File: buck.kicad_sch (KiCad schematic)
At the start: 8 parts, among them U7 DIO6012BCST6

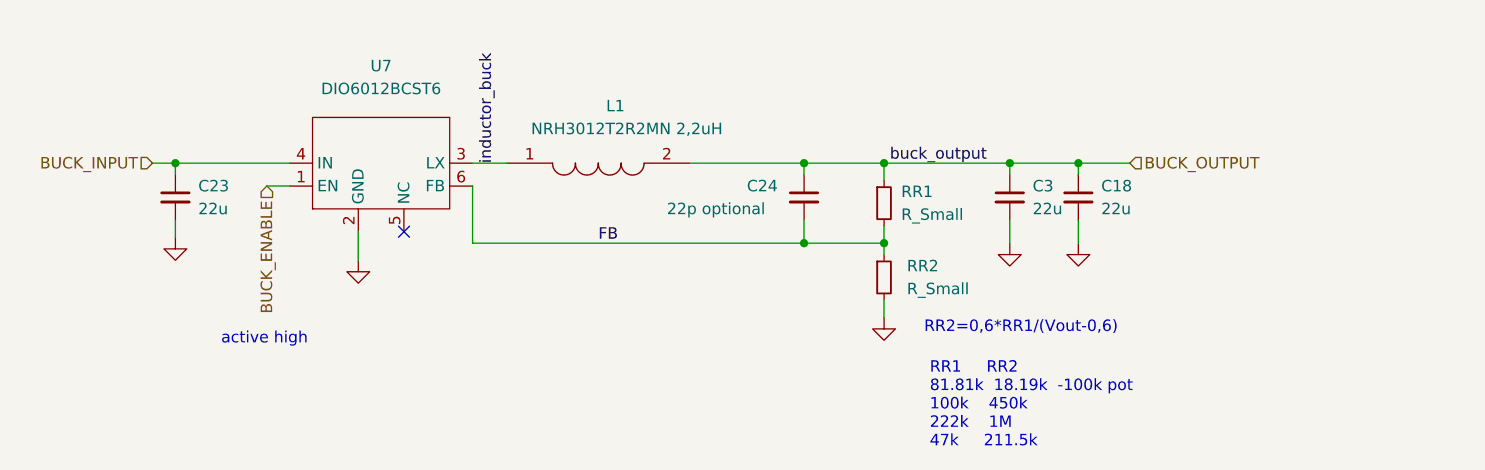
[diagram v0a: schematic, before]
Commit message: j
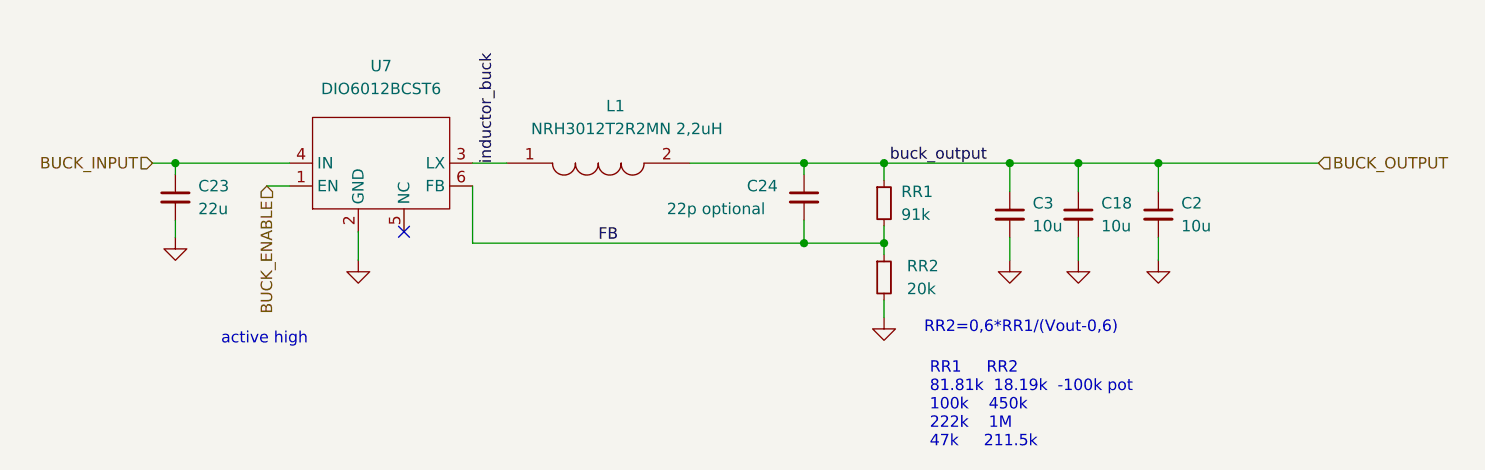
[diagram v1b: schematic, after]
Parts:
- added C2: 10u, Capacitor_SMD:C_0805_2012Metric, symbol Device:C_Small
- C18, C3: value 22u -> 10u; footprint Capacitor_THT:CP_Radial_D5.0mm_P2.00mm -> Capacitor_SMD:C_0805_2012Metric
- RR1: value R_Small -> 91k; footprint Resistor_THT:R_Axial_DIN0204_L3.6mm_D1.6mm_P5.08mm_Vertical -> Resistor_SMD:R_0805_2012Metric
- RR2: value R_Small -> 20k; footprint Resistor_THT:R_Axial_DIN0204_L3.6mm_D1.6mm_P5.08mm_Vertical -> Resistor_SMD:R_0805_2012Metric
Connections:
- net BUCK_OUTPUT: now also C2.1
- net GND: now also C2.2
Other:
- moved on the sheet: C18, C3
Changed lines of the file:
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@@
   (junction (at 83.82 59.69) (diameter 0) (color 0 0 0 0)
+  )
+  (junction (at 193.04 59.69) (diameter 0) (color 0 0 0 0)
   )
   (junction (at 162.56 59.69) (diameter 0) (color 0 0 0 0)
@@
     (stroke (width 0) (type default) (color 0 0 0 0))
   )
-  (wire (pts (xy 184.15 59.69) (xy 184.15 60.96))
+  (wire (pts (xy 184.15 59.69) (xy 184.15 62.865))
     (stroke (width 0) (type default) (color 0 0 0 0))
   )
@@
     (stroke (width 0) (type default) (color 0 0 0 0))
   )
+  (wire (pts (xy 193.04 59.69) (xy 210.82 59.69))
+    (stroke (width 0) (type default) (color 0 0 0 0))
+  )
   (wire (pts (xy 153.67 68.58) (xy 162.56 68.58))
     (stroke (width 0) (type default) (color 0 0 0 0))
   )
-  (wire (pts (xy 176.53 66.04) (xy 176.53 68.58))
+  (wire (pts (xy 176.53 67.945) (xy 176.53 70.485))
     (stroke (width 0) (type default) (color 0 0 0 0))
   )
@@
     (stroke (width 0) (type default) (color 0 0 0 0))
   )
-  (wire (pts (xy 184.15 59.69) (xy 189.865 59.69))
+  (wire (pts (xy 184.15 59.69) (xy 193.04 59.69))
     (stroke (width 0) (type default) (color 0 0 0 0))
   )
@@
     (stroke (width 0) (type default) (color 0 0 0 0))
   )
-  (wire (pts (xy 176.53 59.69) (xy 176.53 60.96))
+  (wire (pts (xy 176.53 59.69) (xy 176.53 62.865))
     (stroke (width 0) (type default) (color 0 0 0 0))
   )
@@
     (stroke (width 0) (type default) (color 0 0 0 0))
   )
+  (wire (pts (xy 193.04 67.945) (xy 193.04 70.485))
+    (stroke (width 0) (type default) (color 0 0 0 0))
+  )
+  (wire (pts (xy 193.04 59.69) (xy 193.04 62.865))
+    (stroke (width 0) (type default) (color 0 0 0 0))
+  )
   (wire (pts (xy 104.14 67.31) (xy 104.14 70.485))
     (stroke (width 0) (type default) (color 0 0 0 0))
@@
     (stroke (width 0) (type default) (color 0 0 0 0))
   )
-  (wire (pts (xy 184.15 66.04) (xy 184.15 68.58))
+  (wire (pts (xy 184.15 67.945) (xy 184.15 70.485))
     (stroke (width 0) (type default) (color 0 0 0 0))
   )
@@
     (effects (font (size 1.27 1.27)) (justify right))
   )
-  (hierarchical_label "BUCK_OUTPUT" (shape input) (at 189.865 59.69 0)
+  (hierarchical_label "BUCK_OUTPUT" (shape input) (at 210.82 59.69 0)
     (effects (font (size 1.27 1.27)) (justify left))
   )
@@
       (effects (font (size 1.27 1.27)) (justify left))
     )
-    (property "Value" "R_Small" (id 1) (at 165.1 73.6599 0)
-      (effects (font (size 1.27 1.27)) (justify left))
-    )
-    (property "Footprint" "Resistor_THT:R_Axial_DIN0204_L3.6mm_D1.6mm_P5.08mm_Vertical" (id 2) (at 162.56 72.39 0)
+    (property "Value" "20k" (id 1) (at 165.1 73.6599 0)
+      (effects (font (size 1.27 1.27)) (justify left))
+    )
+    (property "Footprint" "Resistor_SMD:R_0805_2012Metric" (id 2) (at 162.56 72.39 0)
       (effects (font (size 1.27 1.27)) hide)
     )
@@
     (pin "1")
   )
-  (symbol (lib_id "power:GND") (at 184.15 68.58 0) (unit 1)
-    (in_bom yes) (on_board yes) (fields_autoplaced)
-    (property "Reference" "#PWR0104" (id 0) (at 184.15 74.93 0)
-      (effects (font (size 1.27 1.27)) hide)
-    )
-    (property "Value" "GND" (id 1) (at 184.15 73.66 0)
-      (effects (font (size 1.27 1.27)) hide)
-    )
-    (property "Footprint" "" (id 2) (at 184.15 68.58 0)
-      (effects (font (size 1.27 1.27)) hide)
-    )
-    (property "Datasheet" "" (id 3) (at 184.15 68.58 0)
+  (symbol (lib_id "power:GND") (at 193.04 70.485 0) (unit 1)
+    (in_bom yes) (on_board yes) (fields_autoplaced)
+    (property "Reference" "#PWR071" (id 0) (at 193.04 76.835 0)
+      (effects (font (size 1.27 1.27)) hide)
+    )
+    (property "Value" "GND" (id 1) (at 193.04 75.565 0)
+      (effects (font (size 1.27 1.27)) hide)
+    )
+    (property "Footprint" "" (id 2) (at 193.04 70.485 0)
+      (effects (font (size 1.27 1.27)) hide)
+    )
+    (property "Datasheet" "" (id 3) (at 193.04 70.485 0)
+      (effects (font (size 1.27 1.27)) hide)
+    )
+    (pin "1")
+  )
+  (symbol (lib_name "C_Small_1") (lib_id "Device:C_Small") (at 193.04 65.405 0) (unit 1)
+    (in_bom yes) (on_board yes) (fields_autoplaced)
+    (property "Reference" "C2" (id 0) (at 195.58 64.1412 0)
+      (effects (font (size 1.27 1.27)) (justify left))
+    )
+    (property "Value" "10u" (id 1) (at 195.58 66.6812 0)
+      (effects (font (size 1.27 1.27)) (justify left))
+    )
+    (property "Footprint" "Capacitor_SMD:C_0805_2012Metric" (id 2) (at 193.04 65.405 0)
+      (effects (font (size 1.27 1.27)) hide)
+    )
+    (property "Datasheet" "~" (id 3) (at 193.04 65.405 0)
+      (effects (font (size 1.27 1.27)) hide)
+    )
+    (pin "1")
+    (pin "2")
+  )
+  (symbol (lib_id "power:GND") (at 184.15 70.485 0) (unit 1)
+    (in_bom yes) (on_board yes) (fields_autoplaced)
+    (property "Reference" "#PWR0104" (id 0) (at 184.15 76.835 0)
+      (effects (font (size 1.27 1.27)) hide)
+    )
+    (property "Value" "GND" (id 1) (at 184.15 75.565 0)
+      (effects (font (size 1.27 1.27)) hide)
+    )
+    (property "Footprint" "" (id 2) (at 184.15 70.485 0)
+      (effects (font (size 1.27 1.27)) hide)
+    )
+    (property "Datasheet" "" (id 3) (at 184.15 70.485 0)
       (effects (font (size 1.27 1.27)) hide)
     )
@@
     (pin "2")
   )
-  (symbol (lib_id "power:GND") (at 176.53 68.58 0) (unit 1)
-    (in_bom yes) (on_board yes) (fields_autoplaced)
-    (property "Reference" "#PWR0105" (id 0) (at 176.53 74.93 0)
-      (effects (font (size 1.27 1.27)) hide)
-    )
-    (property "Value" "GND" (id 1) (at 176.53 73.66 0)
-      (effects (font (size 1.27 1.27)) hide)
-    )
-    (property "Footprint" "" (id 2) (at 176.53 68.58 0)
-      (effects (font (size 1.27 1.27)) hide)
-    )
-    (property "Datasheet" "" (id 3) (at 176.53 68.58 0)
+  (symbol (lib_id "power:GND") (at 176.53 70.485 0) (unit 1)
+    (in_bom yes) (on_board yes) (fields_autoplaced)
+    (property "Reference" "#PWR0105" (id 0) (at 176.53 76.835 0)
+      (effects (font (size 1.27 1.27)) hide)
+    )
+    (property "Value" "GND" (id 1) (at 176.53 75.565 0)
+      (effects (font (size 1.27 1.27)) hide)
+    )
+    (property "Footprint" "" (id 2) (at 176.53 70.485 0)
+      (effects (font (size 1.27 1.27)) hide)
+    )
+    (property "Datasheet" "" (id 3) (at 176.53 70.485 0)
       (effects (font (size 1.27 1.27)) hide)
     )
@@
     (pin "2")
   )
-  (symbol (lib_id "Device:C_Small") (at 184.15 63.5 0) (unit 1)
-    (in_bom yes) (on_board yes) (fields_autoplaced)
-    (property "Reference" "C18" (id 0) (at 186.69 62.2362 0)
-      (effects (font (size 1.27 1.27)) (justify left))
-    )
-    (property "Value" "22u" (id 1) (at 186.69 64.7762 0)
-      (effects (font (size 1.27 1.27)) (justify left))
-    )
-    (property "Footprint" "Capacitor_THT:CP_Radial_D5.0mm_P2.00mm" (id 2) (at 184.15 63.5 0)
-      (effects (font (size 1.27 1.27)) hide)
-    )
-    (property "Datasheet" "~" (id 3) (at 184.15 63.5 0)
-      (effects (font (size 1.27 1.27)) hide)
-    )
-    (pin "1")
-    (pin "2")
-  )
-  (symbol (lib_id "Device:C_Small") (at 176.53 63.5 0) (unit 1)
-    (in_bom yes) (on_board yes) (fields_autoplaced)
-    (property "Reference" "C3" (id 0) (at 179.07 62.2362 0)
-      (effects (font (size 1.27 1.27)) (justify left))
-    )
-    (property "Value" "22u" (id 1) (at 179.07 64.7762 0)
-      (effects (font (size 1.27 1.27)) (justify left))
-    )
-    (property "Footprint" "Capacitor_THT:CP_Radial_D5.0mm_P2.00mm" (id 2) (at 176.53 63.5 0)
-      (effects (font (size 1.27 1.27)) hide)
-    )
-    (property "Datasheet" "~" (id 3) (at 176.53 63.5 0)
+  (symbol (lib_id "Device:C_Small") (at 184.15 65.405 0) (unit 1)
+    (in_bom yes) (on_board yes) (fields_autoplaced)
+    (property "Reference" "C18" (id 0) (at 186.69 64.1412 0)
+      (effects (font (size 1.27 1.27)) (justify left))
+    )
+    (property "Value" "10u" (id 1) (at 186.69 66.6812 0)
+      (effects (font (size 1.27 1.27)) (justify left))
+    )
+    (property "Footprint" "Capacitor_SMD:C_0805_2012Metric" (id 2) (at 184.15 65.405 0)
+      (effects (font (size 1.27 1.27)) hide)
+    )
+    (property "Datasheet" "~" (id 3) (at 184.15 65.405 0)
+      (effects (font (size 1.27 1.27)) hide)
+    )
+    (pin "1")
+    (pin "2")
+  )
+  (symbol (lib_name "C_Small_1") (lib_id "Device:C_Small") (at 176.53 65.405 0) (unit 1)
+    (in_bom yes) (on_board yes) (fields_autoplaced)
+    (property "Reference" "C3" (id 0) (at 179.07 64.1412 0)
+      (effects (font (size 1.27 1.27)) (justify left))
+    )
+    (property "Value" "10u" (id 1) (at 179.07 66.6812 0)
+      (effects (font (size 1.27 1.27)) (justify left))
+    )
+    (property "Footprint" "Capacitor_SMD:C_0805_2012Metric" (id 2) (at 176.53 65.405 0)
+      (effects (font (size 1.27 1.27)) hide)
+    )
+    (property "Datasheet" "~" (id 3) (at 176.53 65.405 0)
       (effects (font (size 1.27 1.27)) hide)
     )
@@
       (effects (font (size 1.27 1.27)) (justify left))
     )
-    (property "Value" "R_Small" (id 1) (at 164.465 65.4049 0)
-      (effects (font (size 1.27 1.27)) (justify left))
-    )
-    (property "Footprint" "Resistor_THT:R_Axial_DIN0204_L3.6mm_D1.6mm_P5.08mm_Vertical" (id 2) (at 162.56 64.135 0)
-      (effects (font (size 1.27 1.27)) hide)
-    )
+    (property "Value" "91k" (id 1) (at 164.465 65.4049 0)
+      (effects (font (size 1.27 1.27)) (justify left))
+    )
+    (property "Footprint" "Resistor_SMD:R_0805_2012Metric" (id 2) (at 162.56 64.135 0)
+      (effects (font (size 1.27 1.27)) hide)
+    )
